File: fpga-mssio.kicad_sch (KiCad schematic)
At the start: 14 parts, among them U1 MPFS250T-FCVG484

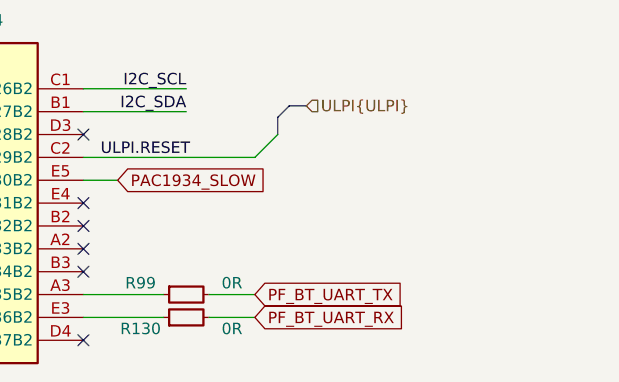
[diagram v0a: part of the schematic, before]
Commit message: [#57505] Finish defining buses
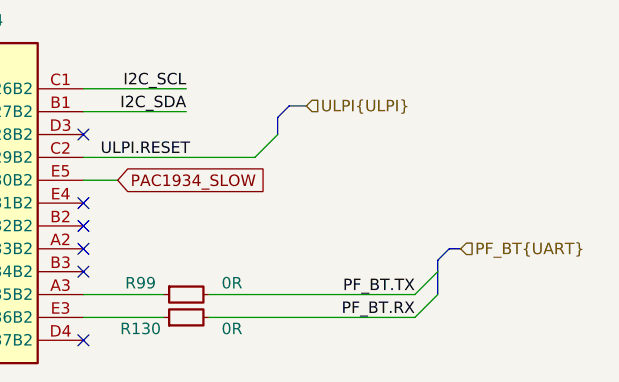
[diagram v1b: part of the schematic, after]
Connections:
- net PF_BT_UART_RX renamed PF_BT.RX
- net PF_BT_UART_TX renamed PF_BT.TX
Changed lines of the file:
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@@
   (no_connect (at 332.105 200.025))
   (no_connect (at 332.105 202.565))
+  (bus_entry (at 368.935 210.185) (size 2.54 -2.54)
+    (stroke (width 0) (type default))
+  )
   (bus_entry (at 189.23 158.75) (size 2.54 -2.54)
     (stroke (width 0) (type default))
@@
     (stroke (width 0) (type default))
   )
+  (bus_entry (at 368.935 212.725) (size 2.54 -2.54)
+    (stroke (width 0) (type default))
+  )
   (bus_entry (at 189.23 147.32) (size 2.54 -2.54)
     (stroke (width 0) (type default))
@@
     (stroke (width 0) (type default))
   )
+  (bus (pts (xy 372.745 205.105) (xy 371.475 206.375))
+    (stroke (width 0) (type default))
+  )
   (wire (pts (xy 304.165 97.155) (xy 301.625 97.155))
     (stroke (width 0) (type default))
@@
     (stroke (width 0) (type default))
   )
+  (bus (pts (xy 371.475 207.645) (xy 371.475 210.185))
+    (stroke (width 0) (type default))
+  )
   (polyline (pts (xy 179.07 78.74) (xy 179.07 91.44))
     (stroke (width 0) (type default))
@@
     (stroke (width 0) (type default))
   )
+  (bus (pts (xy 371.475 206.375) (xy 371.475 207.645))
+    (stroke (width 0) (type default))
+  )
   (wire (pts (xy 158.75 66.04) (xy 198.755 66.04))
     (stroke (width 0) (type default))
@@
     (stroke (width 0) (type default))
   )
-  (wire (pts (xy 346.075 212.725) (xy 351.155 212.725))
+  (wire (pts (xy 346.075 212.725) (xy 368.935 212.725))
     (stroke (width 0) (type default))
   )
@@
     (stroke (width 0) (type default))
   )
-  (wire (pts (xy 346.075 210.185) (xy 351.155 210.185))
+  (wire (pts (xy 346.075 210.185) (xy 368.935 210.185))
     (stroke (width 0) (type default))
   )
@@
   )
   (bus (pts (xy 88.9 142.24) (xy 88.9 144.78))
+    (stroke (width 0) (type default))
+  )
+  (bus (pts (xy 372.745 205.105) (xy 374.015 205.105))
     (stroke (width 0) (type default))
   )
@@
     (effects (font (size 1.27 1.27)) (justify right bottom))
   )
+  (label "PF_BT.RX" (at 368.935 212.725 180) (fields_autoplaced)
+    (effects (font (size 1.27 1.27)) (justify right bottom))
+  )
   (label "SD.DAT3" (at 189.23 139.7 180) (fields_autoplaced)
     (effects (font (size 1.27 1.27)) (justify right bottom))
@@
     (effects (font (size 1.27 1.27)) (justify left bottom))
   )
+  (label "PF_BT.TX" (at 368.935 210.185 180) (fields_autoplaced)
+    (effects (font (size 1.27 1.27)) (justify right bottom))
+  )
   (label "MEM.DAT1" (at 89.535 71.12 0) (fields_autoplaced)
     (effects (font (size 1.27 1.27)) (justify left bottom))
@@
   (label "SD.DAT0" (at 189.23 142.24 180) (fields_autoplaced)
     (effects (font (size 1.27 1.27)) (justify right bottom))
-  )
-  (global_label "PF_BT_UART_TX" (shape input) (at 351.155 210.185 0) (fields_autoplaced)
-    (effects (font (size 1.27 1.27)) (justify left))
-    (property "Intersheetrefs" "${INTERSHEET_REFS}" (at 368.473 210.185 0)
-      (effects (font (size 1.27 1.27)) (justify left))
-    )
   )
   (global_label "PAC1934_SLOW" (shape input) (at 335.915 197.485 0) (fields_autoplaced)
@@
     )
   )
-  (global_label "PF_BT_UART_RX" (shape input) (at 351.155 212.725 0) (fields_autoplaced)
-    (effects (font (size 1.27 1.27)) (justify left))
-    (property "Intersheetrefs" "${INTERSHEET_REFS}" (at 368.7754 212.725 0)
-      (effects (font (size 1.27 1.27)) (justify left))
-    )
-  )
   (hierarchical_label "ID{I^{2}C}" (shape input) (at 330.835 89.535 0) (fields_autoplaced)
     (effects (font (size 1.27 1.27)) (justify left))
   )
+  (hierarchical_label "PF_BT{UART}" (shape input) (at 374.015 205.105 0) (fields_autoplaced)
+    (effects (font (size 1.27 1.27)) (justify left))
+  )
